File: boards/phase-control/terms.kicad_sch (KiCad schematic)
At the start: 105 parts, among them Q28 MMBT5401, Q29 MMBT5401, Q30 MMBT5401, Q31 MMBT5401, Q32 MMBT5401, Q33 MMBT5401, Q34 MMBT5401, Q35 MMBT5401, Q36 MMBT5401, Q37 MMBT5401, Q38 MMBT5401, Q39 MMBT5401, Q74 MMBT5401, Q75 MMBT5401, Q76 MMBT5401, Q77 MMBT5401

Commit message: Add script to export production files.
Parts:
- C19, C20, C21: BOM Value (none) -> 120pF
- C900: BOM Value (none) -> 680pF
- CR43, CR44, CR45, CR46, CR47, CR48, CR49, CR50, CR51, CR52, CR53, CR54, CR55, CR93: value 1N5819WS -> 1N4148WS; BOM Value (none) -> 1N4148WS; LCSC (none) -> C2128
- Q28, Q29, Q30, Q31, Q32, Q33, Q34, Q35, Q36, Q37, Q38, Q39, Q74, Q75, Q76, Q77: BOM Value (none) -> MMBT5401; LCSC (none) -> C8326
- R148, R149, R150, R151, R152, R153, R154, R155, R156, R157, R158, R159, R160, R161, R162, R163, R164, R165, R166, R167, R168, R169, R170, R171, R172, R173, R174, R175, R176, R177, R178, R179, R180, R181, R386, R900: BOM Value (none) -> 15kΩ
- R202, R204, R206, R208, R210, R212, R214, R216, R218, R220, R222, R224: BOM Value (none) -> 56kΩ
- R203, R205, R207, R209, R211, R213, R215, R217, R219, R221, R223, R225: BOM Value (none) -> 2kΩ 500mW
- R345, R346, R347: BOM Value (none) -> 6.8kΩ
- R375, R378: BOM Value (none) -> 10kΩ 500mW
- R376, R379, R380: BOM Value (none) -> 33kΩ
- R377, R381: BOM Value (none) -> 800Ω 2W
- R382: BOM Value (none) -> 300Ω 3W

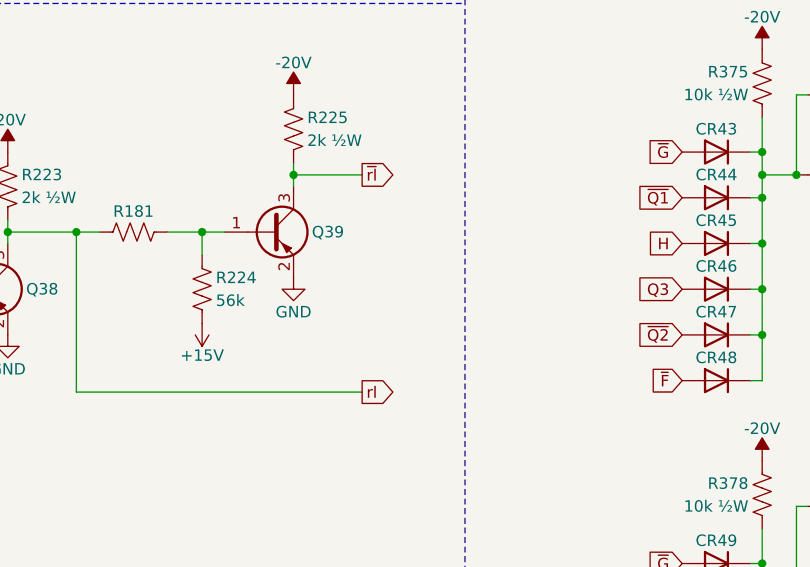
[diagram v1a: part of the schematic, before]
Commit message: Rough layout for Phase Control.
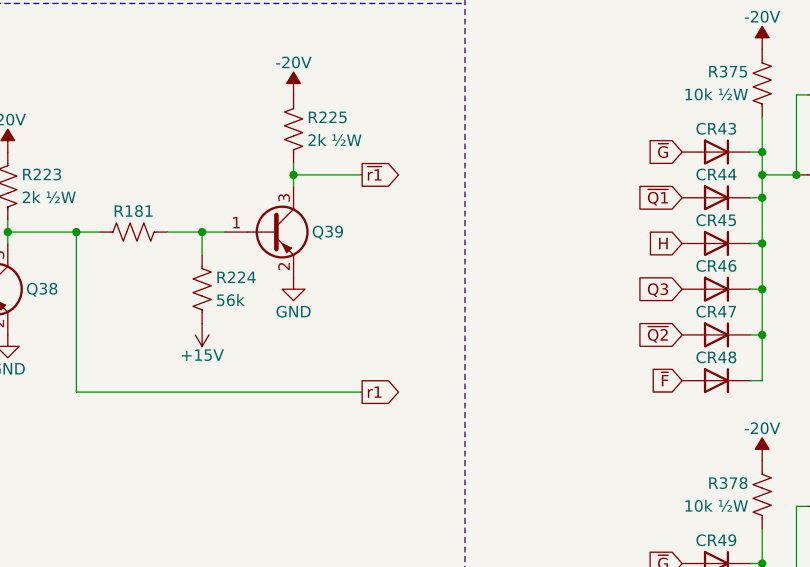
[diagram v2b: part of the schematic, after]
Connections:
- net rl renamed r1
- net ~{rl} renamed ~{r1}
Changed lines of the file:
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@@
 		)
 	)
-	(global_label "~{rl}"
+	(global_label "~{r1}"
 		(shape output)
 		(at 140.97 111.76 0)
@@
 		)
 	)
-	(global_label "rl"
+	(global_label "r1"
 		(shape output)
 		(at 140.97 135.89 0)
